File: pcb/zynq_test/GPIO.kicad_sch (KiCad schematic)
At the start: 0 parts

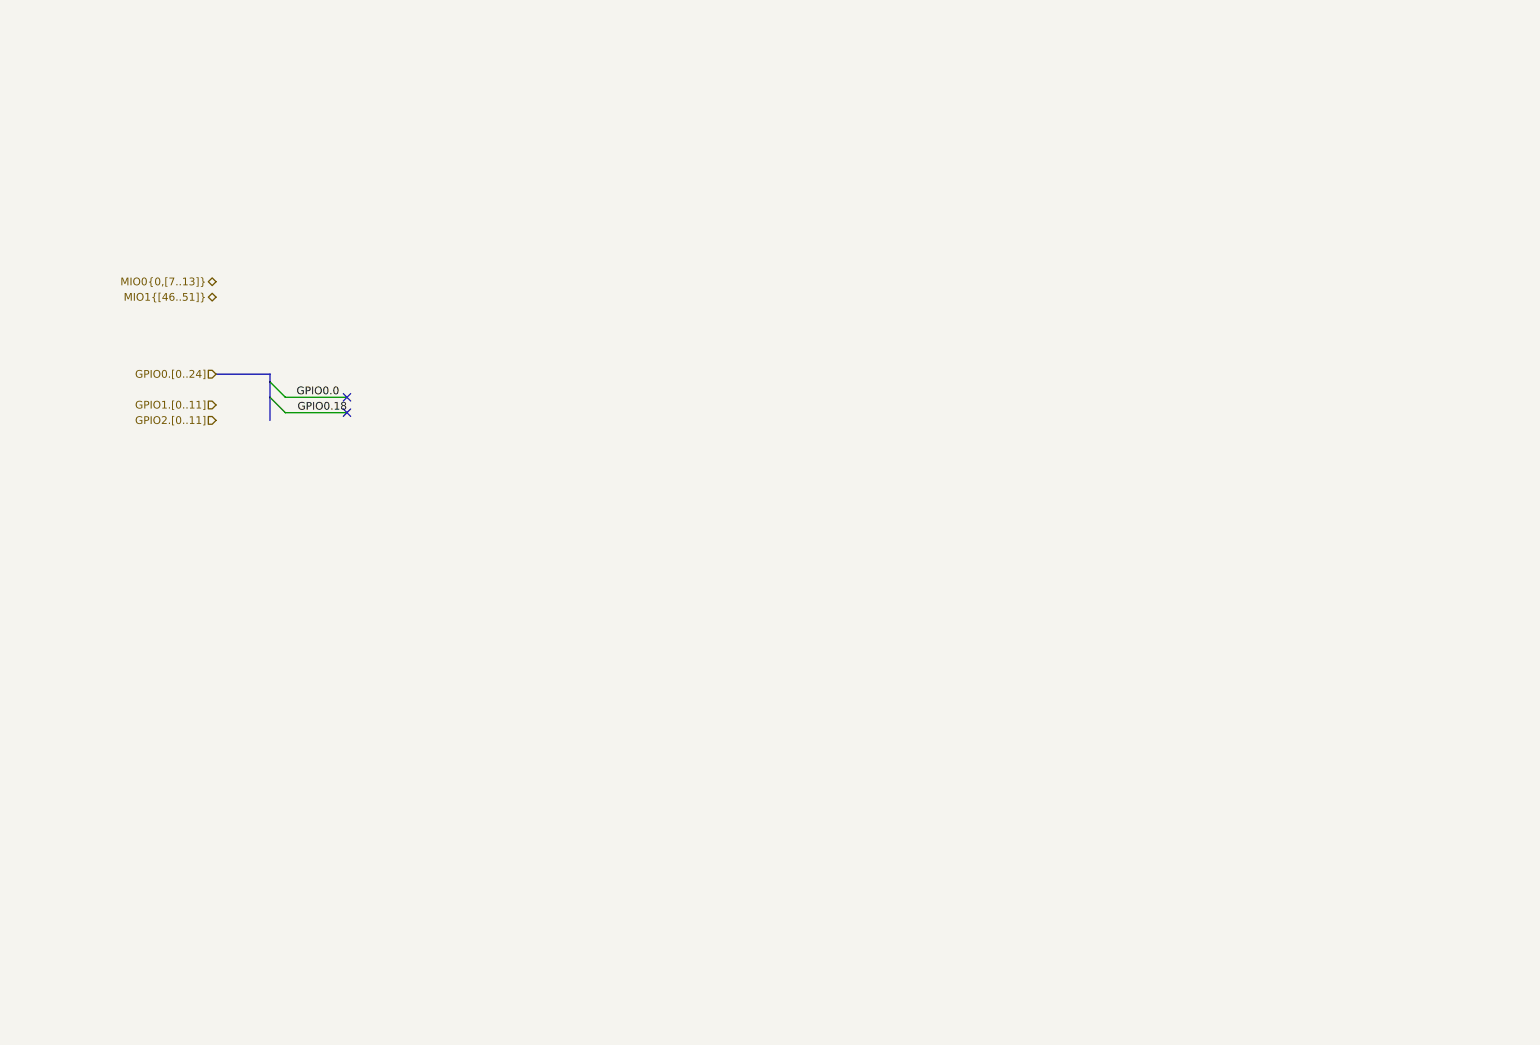
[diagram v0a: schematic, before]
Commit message: Almost done with BOM
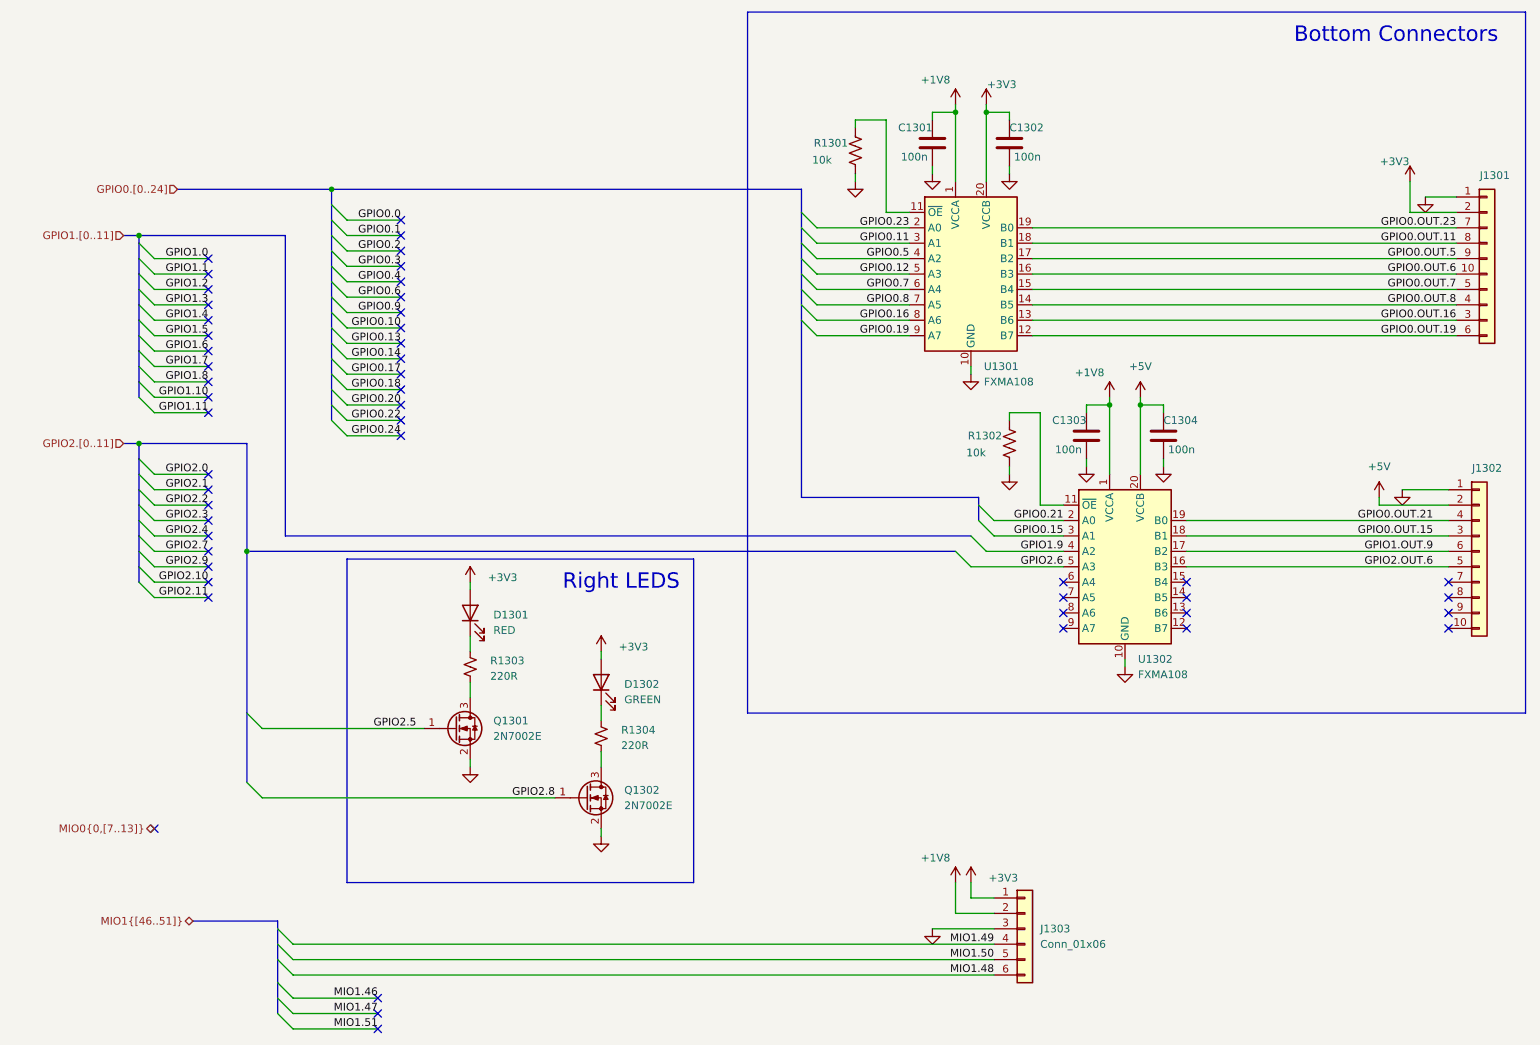
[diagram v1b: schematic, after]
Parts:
- added C1301, C1302, C1303, C1304: 100n, Capacitor_SMD:C_0402_1005Metric, symbol Device:C
- added D1301: RED, LED_SMD:LED_0805_2012Metric, symbol Device:LED
- added D1302: GREEN, LED_SMD:LED_0805_2012Metric, symbol Device:LED
- added J1301, J1302: Conn_02x05_Odd_Even, Connector_PinSocket_2.54mm:PinSocket_2x05_P2.54mm_Horizontal, symbol Connector_Generic:Conn_01x10
- added J1303: Conn_01x06, Connector_PinHeader_2.54mm:PinHeader_1x06_P2.54mm_Vertical, symbol Connector_Generic:Conn_01x06
- added Q1301, Q1302: 2N7002E, Package_TO_SOT_SMD:SOT-23, symbol Transistor_FET:2N7002E
- added R1301, R1302: 10k, Resistor_SMD:R_0402_1005Metric, symbol Device:R_US
- added R1303, R1304: 220R, Resistor_SMD:R_0402_1005Metric, symbol Device:R_Small_US
- added U1301, U1302: FXMA108, Package_DFN_QFN:WQFN-20-1EP_2.5x4.5mm_P0.5mm_EP1x2.9mm, symbol Logic_LevelTranslator:FXMA108
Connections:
- new net: R1302.1, U1302.11 (~{OE})
- new net: D1302.1 (K), R1304.1
- new net: D1301.1 (K), R1303.1
- new net: Q1301.3 (D), R1303.2
- new net: R1301.1, U1301.11 (~{OE})
- new net: Q1302.3 (D), R1304.2
- new net +1V8: C1301.1, C1303.1, J1303.2 (Pin_2), U1301.1 (VCCA), U1302.1 (VCCA)
- new net +3V3: C1302.1, D1301.2 (A), D1302.2 (A), J1301.2 (Pin_2), J1303.1 (Pin_1), U1301.20 (VCCB)
- new net +5V: C1304.1, J1302.2 (Pin_2), U1302.20 (VCCB)
- new net GND: C1301.2, C1302.2, C1303.2, C1304.2, J1301.1 (Pin_1), J1302.1 (Pin_1), J1303.3 (Pin_3), Q1301.2 (S), Q1302.2 (S), R1301.2, R1302.2, U1301.10 (GND), U1302.10 (GND)
- new net GPIO0.11: U1301.3 (A1)
- new net GPIO0.12: U1301.5 (A3)
- new net GPIO0.15: U1302.3 (A1)
- new net GPIO0.16: U1301.8 (A6)
- new net GPIO0.19: U1301.9 (A7)
- new net GPIO0.21: U1302.2 (A0)
- new net GPIO0.23: U1301.2 (A0)
- new net GPIO0.5: U1301.4 (A2)
- new net GPIO0.7: U1301.6 (A4)
- new net GPIO0.8: U1301.7 (A5)
- new net GPIO0.OUT.11: J1301.8 (Pin_8), U1301.18 (B1)
- new net GPIO0.OUT.15: J1302.3 (Pin_3), U1302.18 (B1)
- new net GPIO0.OUT.16: J1301.3 (Pin_3), U1301.13 (B6)
- new net GPIO0.OUT.19: J1301.6 (Pin_6), U1301.12 (B7)
- new net GPIO0.OUT.21: J1302.4 (Pin_4), U1302.19 (B0)
- new net GPIO0.OUT.23: J1301.7 (Pin_7), U1301.19 (B0)
- new net GPIO0.OUT.5: J1301.9 (Pin_9), U1301.17 (B2)
- new net GPIO0.OUT.6: J1301.10 (Pin_10), U1301.16 (B3)
- new net GPIO0.OUT.7: J1301.5 (Pin_5), U1301.15 (B4)
- new net GPIO0.OUT.8: J1301.4 (Pin_4), U1301.14 (B5)
- new net GPIO1.9: U1302.4 (A2)
- new net GPIO1.OUT.9: J1302.6 (Pin_6), U1302.17 (B2)
- new net GPIO2.5: Q1301.1 (G)
- new net GPIO2.6: U1302.5 (A3)
- new net GPIO2.8: Q1302.1 (G)
- new net GPIO2.OUT.6: J1302.5 (Pin_5), U1302.16 (B3)
- new net MIO1.48: J1303.6 (Pin_6)
- new net MIO1.49: J1303.4 (Pin_4)
- new net MIO1.50: J1303.5 (Pin_5)
- no-connect marks 2 -> 51
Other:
- note added: "Bottom Connectors"
- note added: "Right LEDS"

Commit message: Version sent to JLCPCB
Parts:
- C1301, C1302, C1303, C1304: JLCPCB Part# (none) -> C1525; PART_NUMBER (none) -> CL05B104KO5NNNC
- D1301: JLCPCB Part# (none) -> C84256; PART_NUMBER (none) -> NCD0805R1
- D1302: JLCPCB Part# (none) -> C192672; PART_NUMBER (none) -> TJ-S2012SW8TGLC7K-A5
- J1301, J1302, J1303: now left out of the parts list
- Q1301, Q1302: JLCPCB Part# (none) -> C71533; PART_NUMBER (none) -> 2N7002E
- R1301, R1302: JLCPCB Part# (none) -> C191123; PART_NUMBER (none) -> ERJ2RKF1002X
- R1303, R1304: JLCPCB Part# (none) -> C412979; PART_NUMBER (none) -> ERJ2GEJ221X
- U1301, U1302: JLCPCB Part# (none) -> C891320; PART_NUMBER (none) -> FXMA108BQX
